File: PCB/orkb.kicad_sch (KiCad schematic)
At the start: 76 parts, among them J1 USB_C_Receptacle_USB2.0, P1 OLED, SW1 MXHS, SW10 MXHS, SW11 MXHS, SW12 MXHS, SW13 MXHS, SW14 MXHS, SW15 MXHS, SW16 MXHS, SW17 MXHS, SW18 MXHS, SW19 MXHS, SW2 MXHS, SW20 MXHS, SW21 MXHS, SW3 MXHS, SW4 MXHS, SW5 MXHS, SW6 MXHS, SW7 MXHS, SW8 MXHS, SW9 MXHS, U1 ProMicro, U2 SRV05-4, U3 SRV05-4

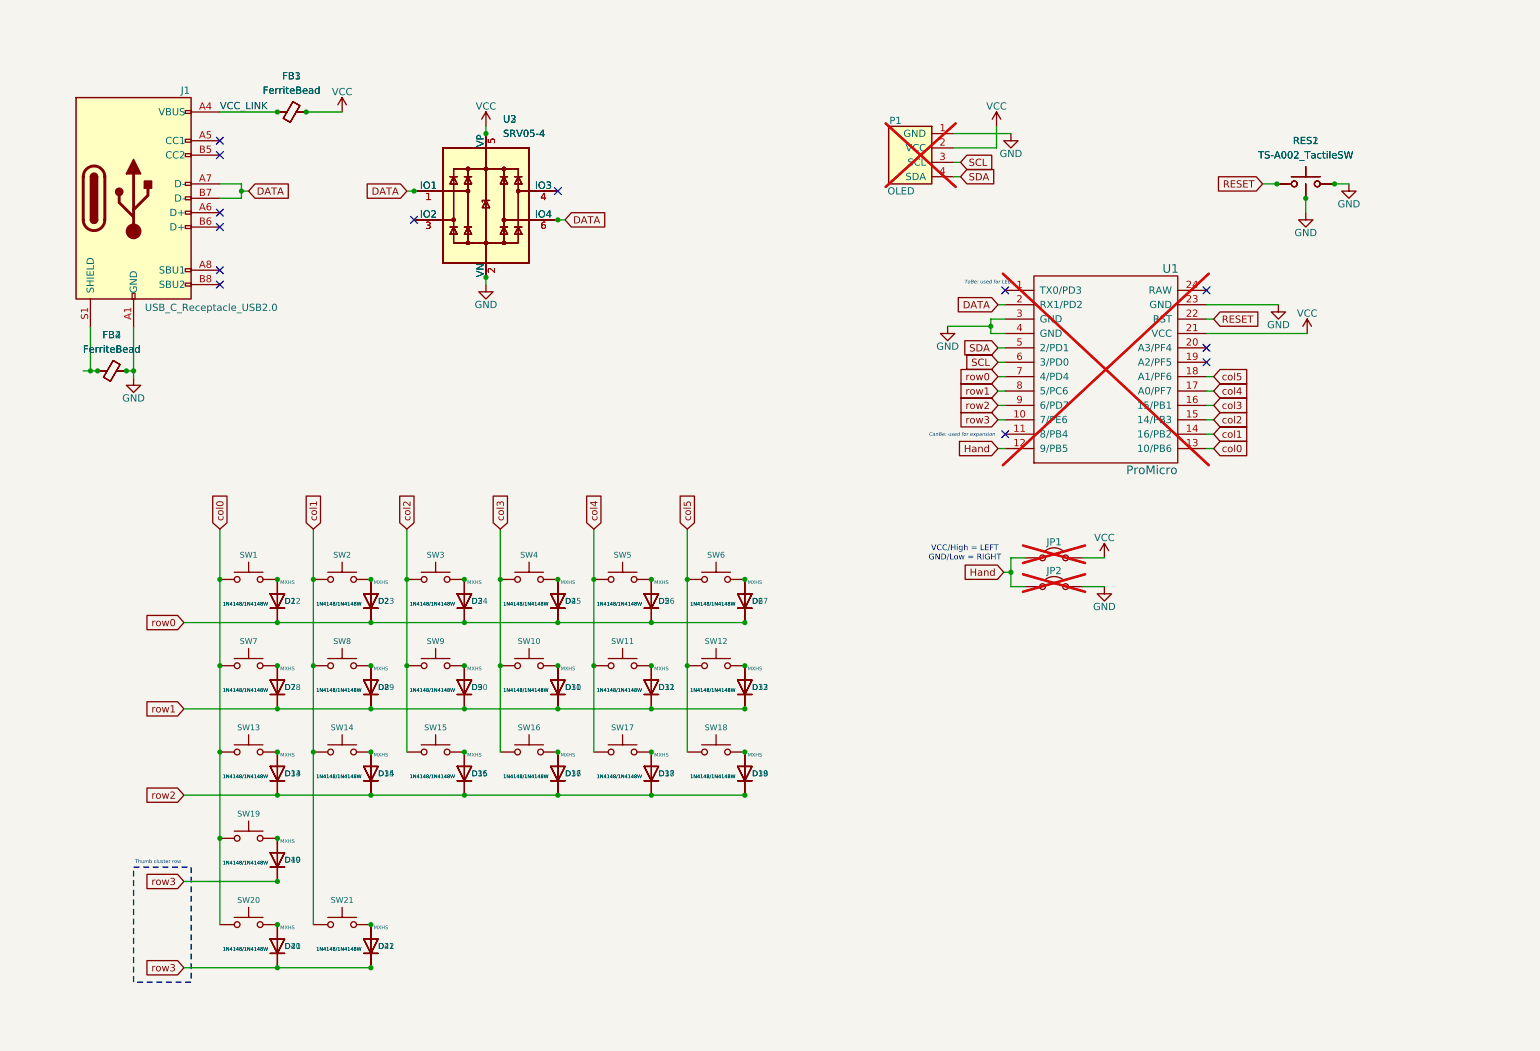
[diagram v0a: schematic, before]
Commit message: Refactoring entire project
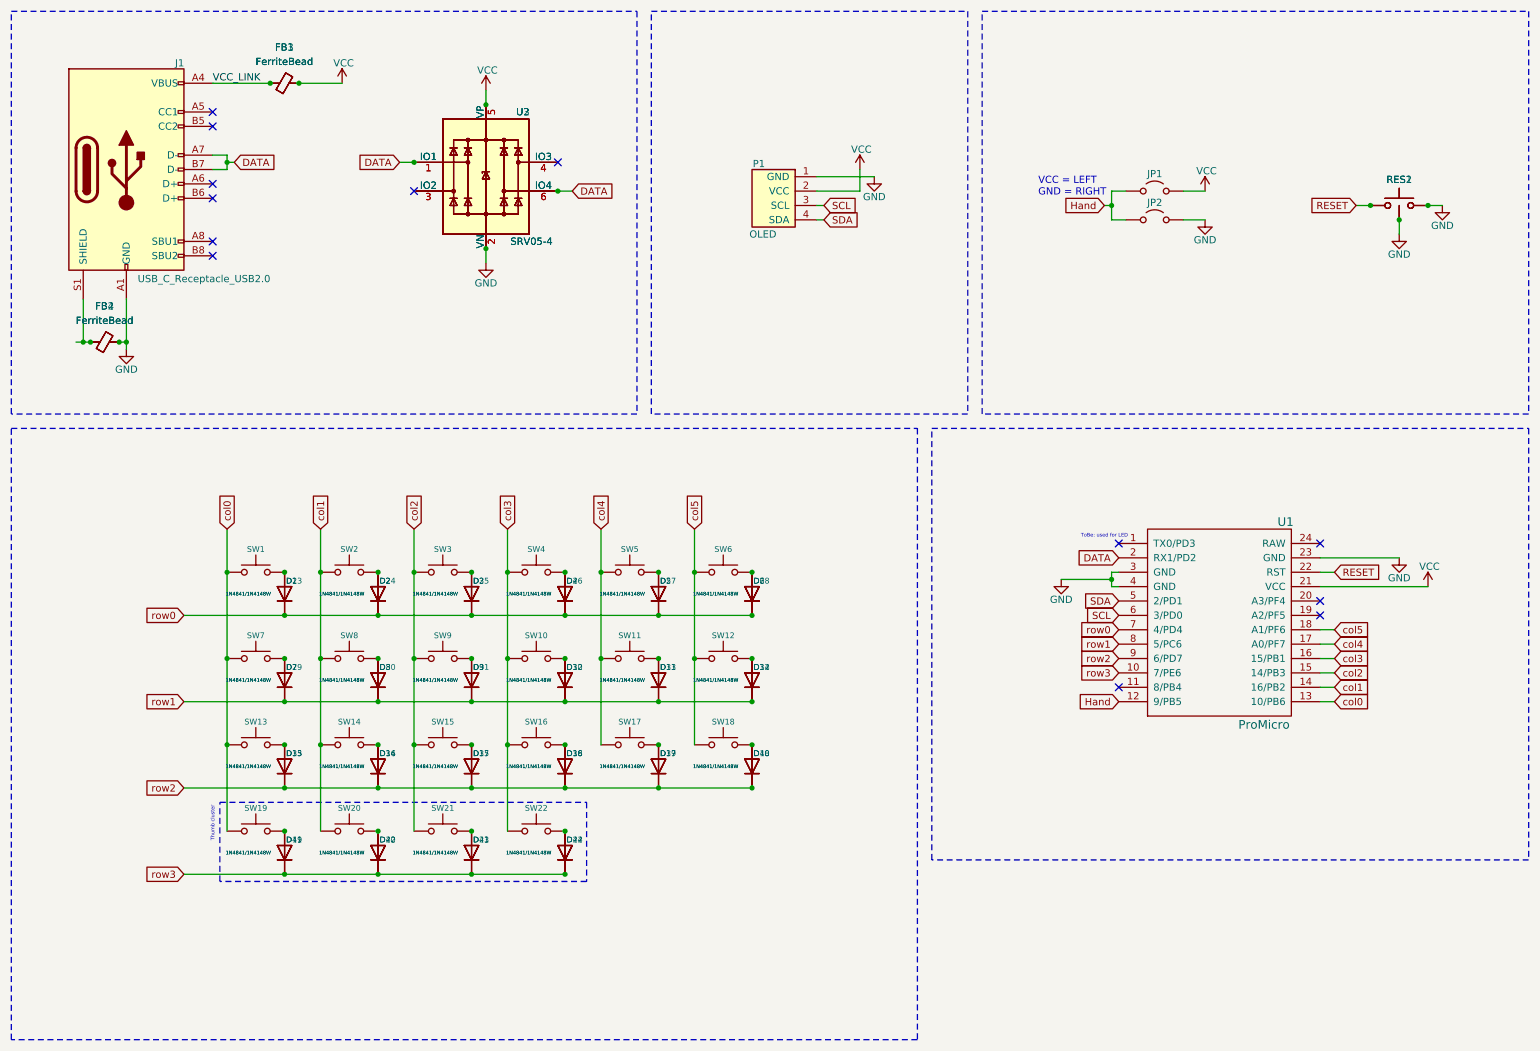
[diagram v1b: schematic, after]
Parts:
- added D43, D44: 1N4841/1N4148W, SplitKeyboard_Common:Diode_DO35_SOD123_Hybrid, symbol Device:D
- added SW22: MXHS, SplitKeyboard_Common:SW_MX_HotSwap_Reversible, symbol Switch:SW_Push
- D1, D10, D11, D12, D13, D14, D15, D16, D17, D18, D19, D2, D20, D21, D22, D23, D24, D25, D26, D27, D28, D29, D3, D30, D31, D32, D33, D34, D35, D36, D37, D38, D39, D4, D40, D41, D42, D5, D6, D7, D8, D9: value 1N4148/1N4148W -> 1N4841/1N4148W
- JP1, JP2: value Jumper_2 -> Jumper_2_Open; footprint Jumper:SolderJumper-2_P1.3mm_Open_TrianglePad1.0x1.5mm -> SplitKeyboard_Common:Jumper_min_v2; now fitted
- P1, U1: now fitted
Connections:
- net col0: no longer SW20.1
- net col1: now also SW20.1; no longer SW21.1
- net col2: now also SW21.1
- net col3: now also SW22.1
- net row0: now also D28.1 (K); no longer D22.1 (K)
- net row1: now also D34.1 (K); no longer D28.1 (K)
- net row2: now also D40.1 (K); no longer D34.1 (K)
- net row3: now also D22.1 (K), D43.1 (K), D44.1 (K); no longer D40.1 (K)
- net at D1.2 (A), SW1.2: now also D23.2 (A); no longer D22.2 (A)
- net at D19.2 (A), SW19.2: now also D41.2 (A); no longer D40.2 (A)
- net at D18.2 (A), SW18.2: now also D40.2 (A); no longer D39.2 (A)
- net at D14.2 (A), SW14.2: now also D36.2 (A); no longer D35.2 (A)
- net at D2.2 (A), SW2.2: now also D24.2 (A); no longer D23.2 (A)
- net at D17.2 (A), SW17.2: now also D39.2 (A); no longer D38.2 (A)
- net at D13.2 (A), SW13.2: now also D35.2 (A); no longer D34.2 (A)
- net at D7.2 (A), SW7.2: now also D29.2 (A); no longer D28.2 (A)
- net at D12.2 (A), SW12.2: now also D34.2 (A); no longer D33.2 (A)
- net at D15.2 (A), SW15.2: now also D37.2 (A); no longer D36.2 (A)
- net at D4.2 (A), SW4.2: now also D26.2 (A); no longer D25.2 (A)
- net at D16.2 (A), SW16.2: now also D38.2 (A); no longer D37.2 (A)
- net at D11.2 (A), SW11.2: now also D33.2 (A); no longer D32.2 (A)
- net at D20.2 (A), SW20.2: now also D42.2 (A); no longer D41.2 (A)
- net at D10.2 (A), SW10.2: now also D32.2 (A); no longer D31.2 (A)
- net at D21.2 (A), SW21.2: now also D43.2 (A); no longer D42.2 (A)
- net at D6.2 (A), SW6.2: now also D28.2 (A); no longer D27.2 (A)
- net at D5.2 (A), SW5.2: now also D27.2 (A); no longer D26.2 (A)
- net at D9.2 (A), SW9.2: now also D31.2 (A); no longer D30.2 (A)
- net at D8.2 (A), SW8.2: now also D30.2 (A); no longer D29.2 (A)
- net at D3.2 (A), SW3.2: now also D25.2 (A); no longer D24.2 (A)
- new net: D22.2 (A), D44.2 (A), SW22.2
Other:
- note added: "Thumb cluster"
- note added: "VCC = LEFT GND = RIGHT"
- note removed: "CanBe: used for expansion"
- note removed: "Thumb cluster row"
- note removed: "VCC/High = LEFT GND/Low = RIGHT"
